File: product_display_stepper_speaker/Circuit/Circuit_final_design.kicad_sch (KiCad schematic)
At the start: 18 parts, among them J1 Barrel_Jack_MountingPin, U1 ESP-12E, U2 LM2931-3.3_TO220, U3 L7805

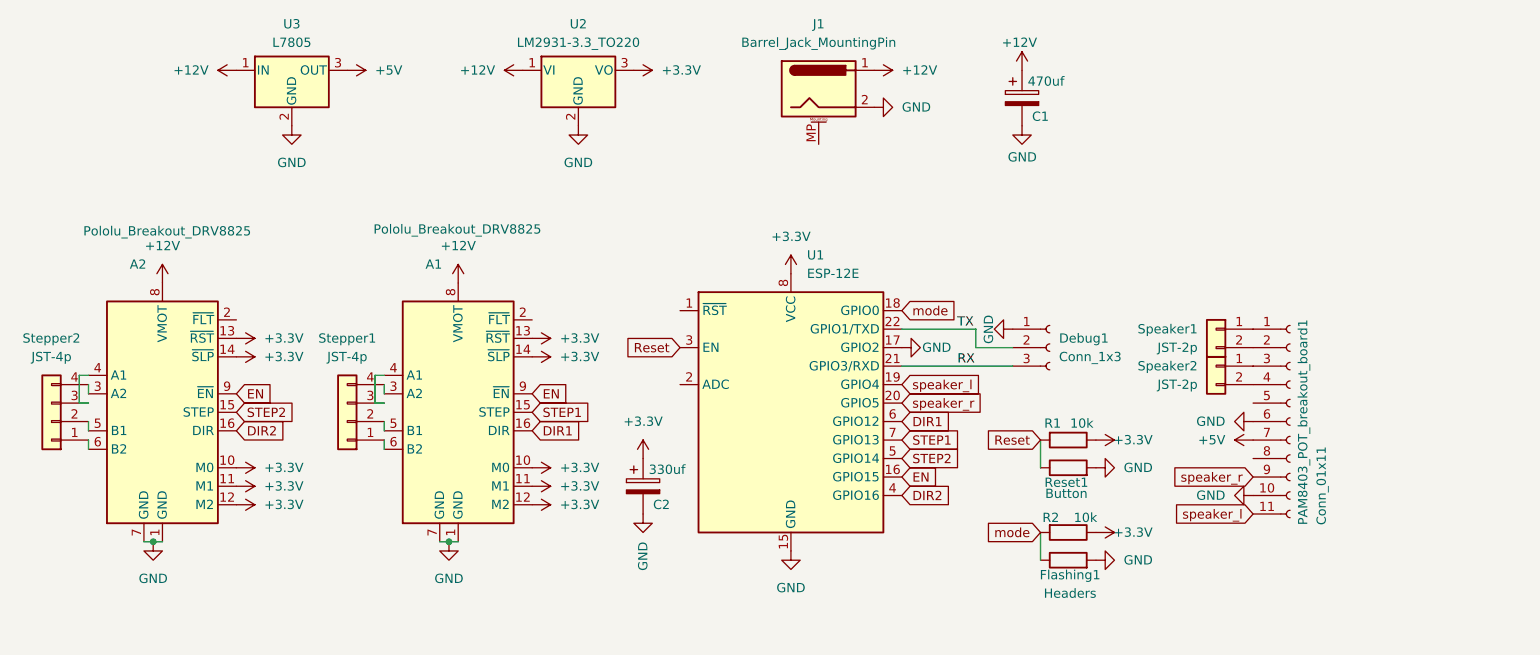
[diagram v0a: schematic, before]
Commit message: finished pcb layout
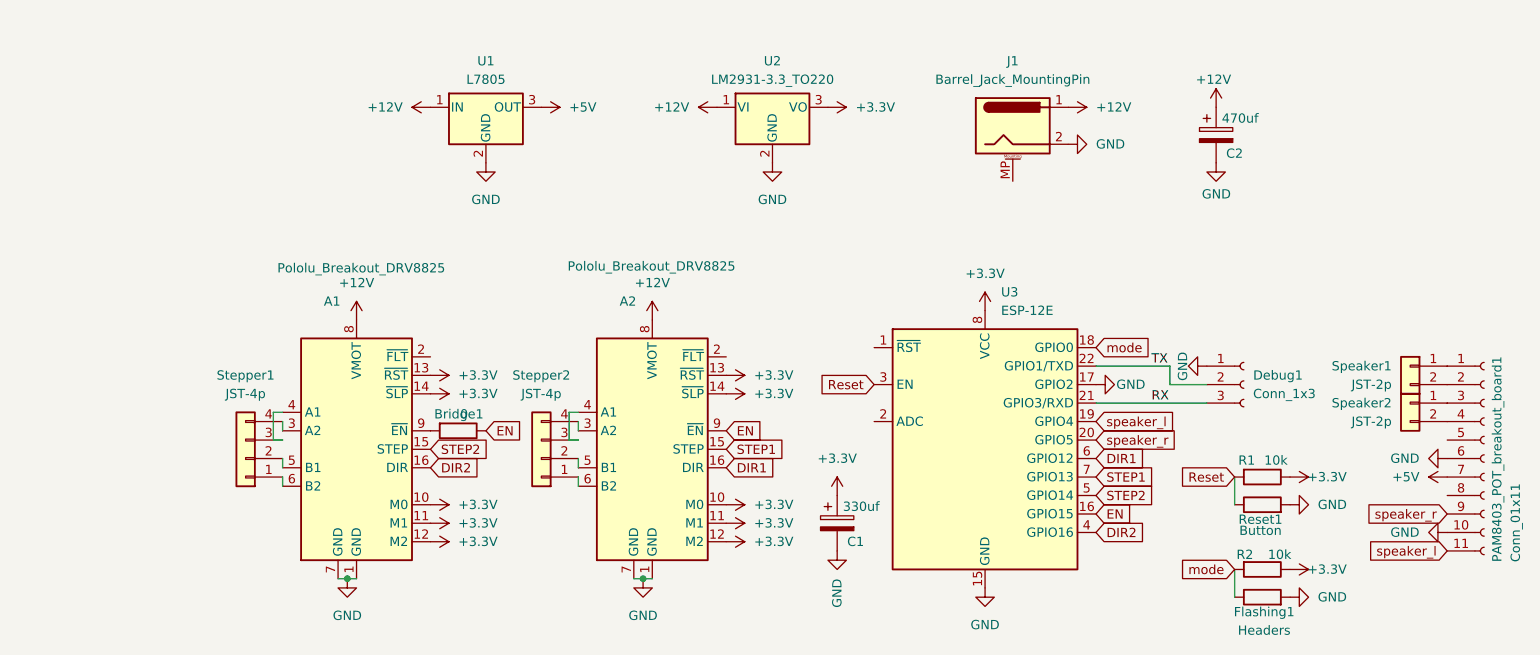
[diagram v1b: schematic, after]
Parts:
- removed U1: ESP-12E, ESP:ESP-12E-DIP, symbol RF_Module:ESP-12E
- removed U3: L7805, Package_TO_SOT_THT:TO-220-3_Vertical, symbol Regulator_Linear:L7805
- added Bridge1: 0, Resistor_THT:R_Axial_DIN0207_L6.3mm_D2.5mm_P7.62mm_Horizontal, symbol Device:R
- added U1: L7805, Package_TO_SOT_THT:TO-220-3_Vertical, symbol Regulator_Linear:L7805
- added U3: ESP-12E, ESP:ESP-12E-DIP, symbol RF_Module:ESP-12E
- C1: value 470uf -> 330uf
- C2: value 330uf -> 470uf
- R1: footprint Resistor_THT:R_Axial_DIN0207_L6.3mm_D2.5mm_P7.62mm_Horizontal -> Resistor_THT:R_Axial_DIN0207_L6.3mm_D2.5mm_P5.08mm_Vertical
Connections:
- net +12V: now also C2.1, U1.1 (IN); no longer C1.1
- net +3.3V: now also C1.1, U3.8 (VCC); no longer C2.1
- net +5V: now also U1.3 (OUT)
- net DIR1: now also A2.16 (DIR), U3.6 (GPIO12); no longer A1.16 (DIR)
- net DIR2: now also A1.16 (DIR), U3.4 (GPIO16); no longer A2.16 (DIR)
- net EN: now also Bridge1.1, U3.16 (GPIO15); no longer A1.9 (~{EN})
- net GND: now also U1.2 (GND), U3.15 (GND), U3.17 (GPIO2)
- net RX: now also U3.21 (GPIO3/RXD)
- net Reset: now also U3.3 (EN)
- net STEP1: now also A2.15 (STEP), U3.7 (GPIO13); no longer A1.15 (STEP)
- net STEP2: now also A1.15 (STEP), U3.5 (GPIO14); no longer A2.15 (STEP)
- net TX: now also U3.22 (GPIO1/TXD)
- net mode: now also U3.18 (GPIO0)
- net speaker_l: now also U3.19 (GPIO4)
- net speaker_r: now also U3.20 (GPIO5)
- new net: A1.9 (~{EN}), Bridge1.2
